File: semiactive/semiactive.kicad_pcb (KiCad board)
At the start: 2 copper layers, 86.6 x 100.8 mm, 2 parts, among them J4 5223002-2, U1 Teensy4.1

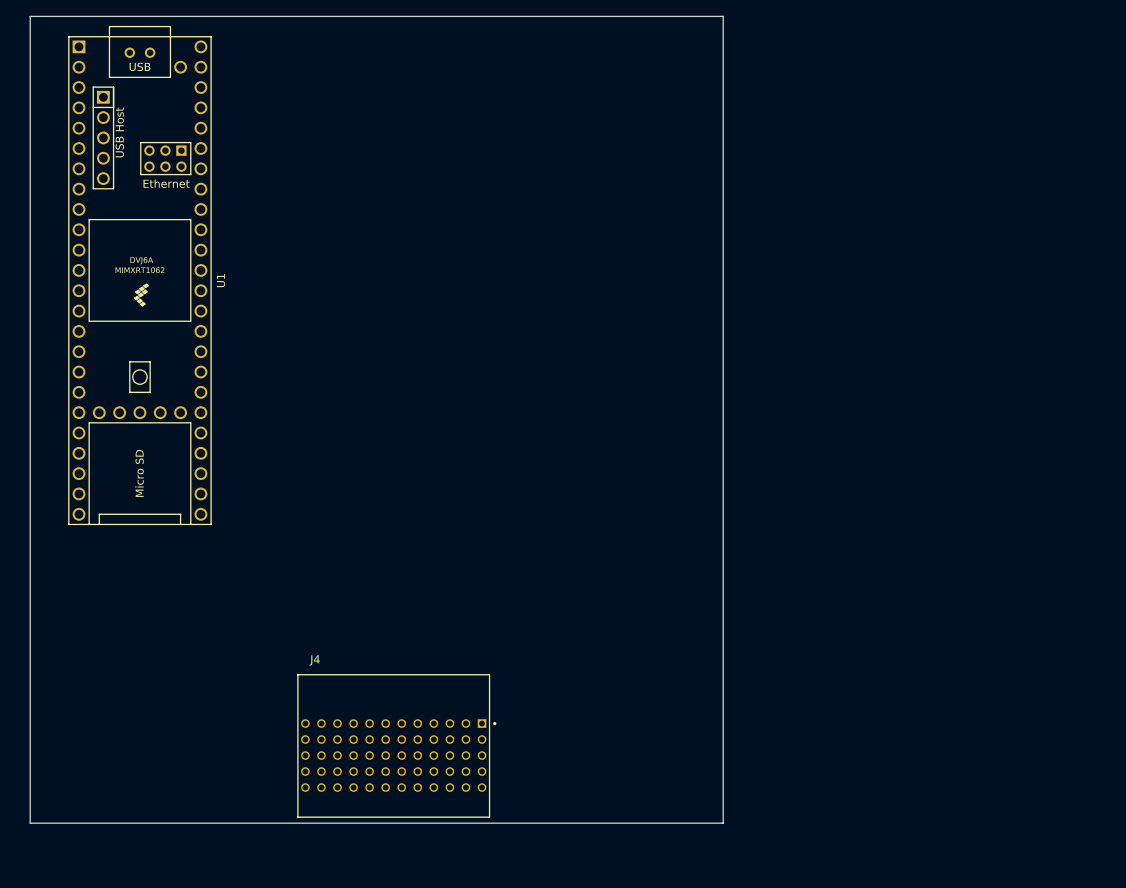
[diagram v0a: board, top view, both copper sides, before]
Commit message: Create a few projects
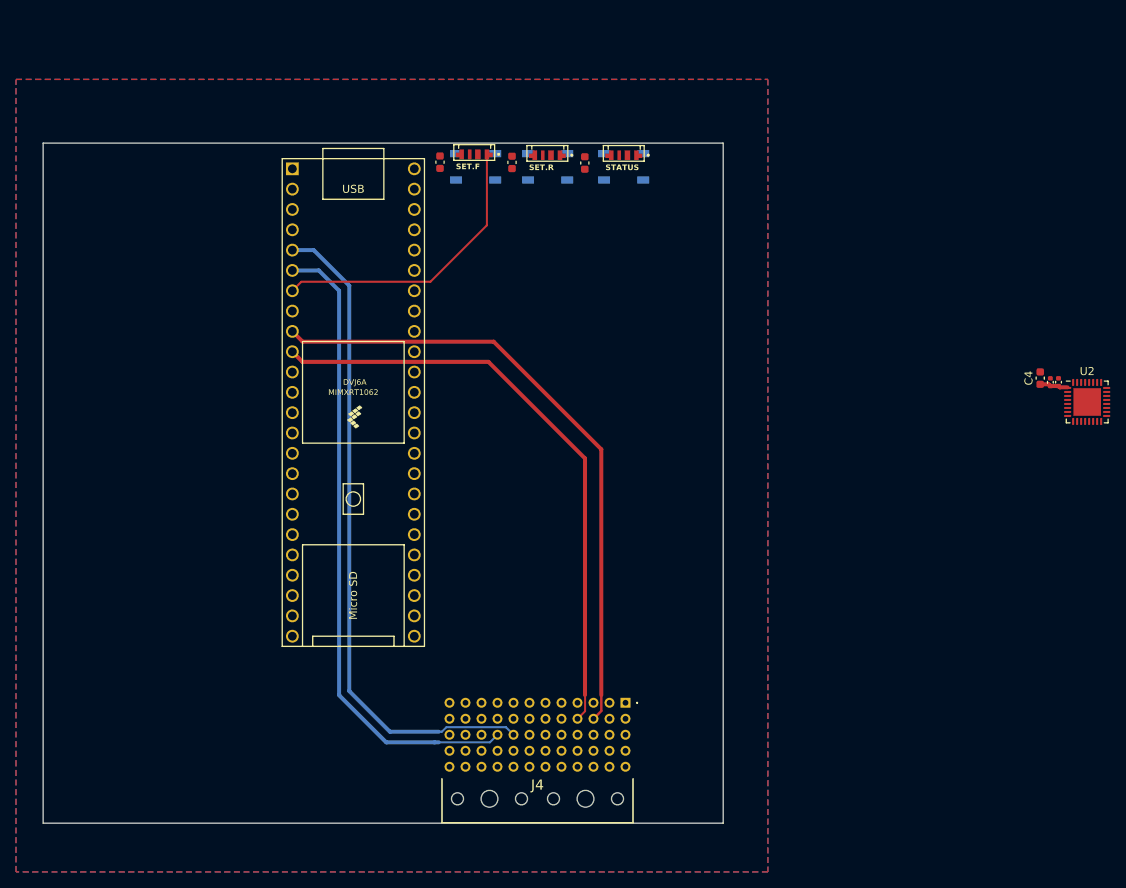
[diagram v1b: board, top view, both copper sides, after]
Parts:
- added C1: C, Capacitor_SMD:C_0603_1608Metric, F.Cu at (164.2, 43.6)
- added C2: C, Capacitor_SMD:C_0603_1608Metric, F.Cu at (173.2, 43.6)
- added C3: C, Capacitor_SMD:C_0603_1608Metric, F.Cu at (182.3, 43.7)
- added C4: 10uF, Capacitor_SMD:C_0603_1608Metric, F.Cu at (239.3, 70.6)
- added C6: .1uF, Capacitor_SMD:C_0402_1005Metric, F.Cu at (241.6, 71.1)
- added C7: 1uF, Capacitor_SMD:C_0402_1005Metric, F.Cu at (240.5, 71.1)
- added D1: SET.F, !footprints:LED_IN-PI42TASPRPGPB, F.Cu at (168.6, 42.5)
- added D2: SET.R, !footprints:LED_IN-PI42TASPRPGPB, F.Cu at (177.8, 42.6)
- added D3: STATUS, !footprints:LED_IN-PI42TASPRPGPB, F.Cu at (187.3, 42.6)
- added D4: SET.F, !footprints:LED_WS2812B_PLCC4_5.0x5.0mm_P3.2mm, B.Cu at (168.7, 44.2)
- added D5: SET.R, !footprints:LED_WS2812B_PLCC4_5.0x5.0mm_P3.2mm, B.Cu at (177.7, 44.2)
- added D6: STATUS, !footprints:LED_WS2812B_PLCC4_5.0x5.0mm_P3.2mm, B.Cu at (187.2, 44.2)
- added U2: ESP8266EX, Package_DFN_QFN:QFN-32-1EP_5x5mm_P0.5mm_EP3.45x3.45mm, F.Cu at (245.1, 73.6)
- J4: footprint 5223002-2:TE_5223002-2 -> !footprints:52230042
- U1: footprint teensy:Teensy41 -> !footprints:Teensy41
- moved U1 30.7 mm to (153.4, 73.7)
- moved J4 18.1 mm to (187.4, 111.2)
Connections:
- U1 pad 7: unconnected-(U1-Pad7) -> ARGBLED
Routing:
- net VOLT1: track 0.00 -> 82.9 mm
- net VOLT2: track 0.00 -> 80.6 mm
- net TX: track 0.00 -> 78.8 mm
- net RX: track 0.00 -> 75.5 mm
- net ARGBLED: track 0.00 -> 36.6 mm
- net 5V: track 0.00 -> 3.59 mm
- added copper zone on B.Cu, net GND
- added copper zone on F.Cu, net GND
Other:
- board size 86.6 x 100.8 mm -> 85 x 85 mm
